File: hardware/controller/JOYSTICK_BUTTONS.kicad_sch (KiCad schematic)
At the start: 14 parts, among them J2 Joystick, J3 Joystick, SW1 UP, SW2 LEFT, SW3 DOWN, SW4 RGHT, SW5 BOOT, SW6 RESET

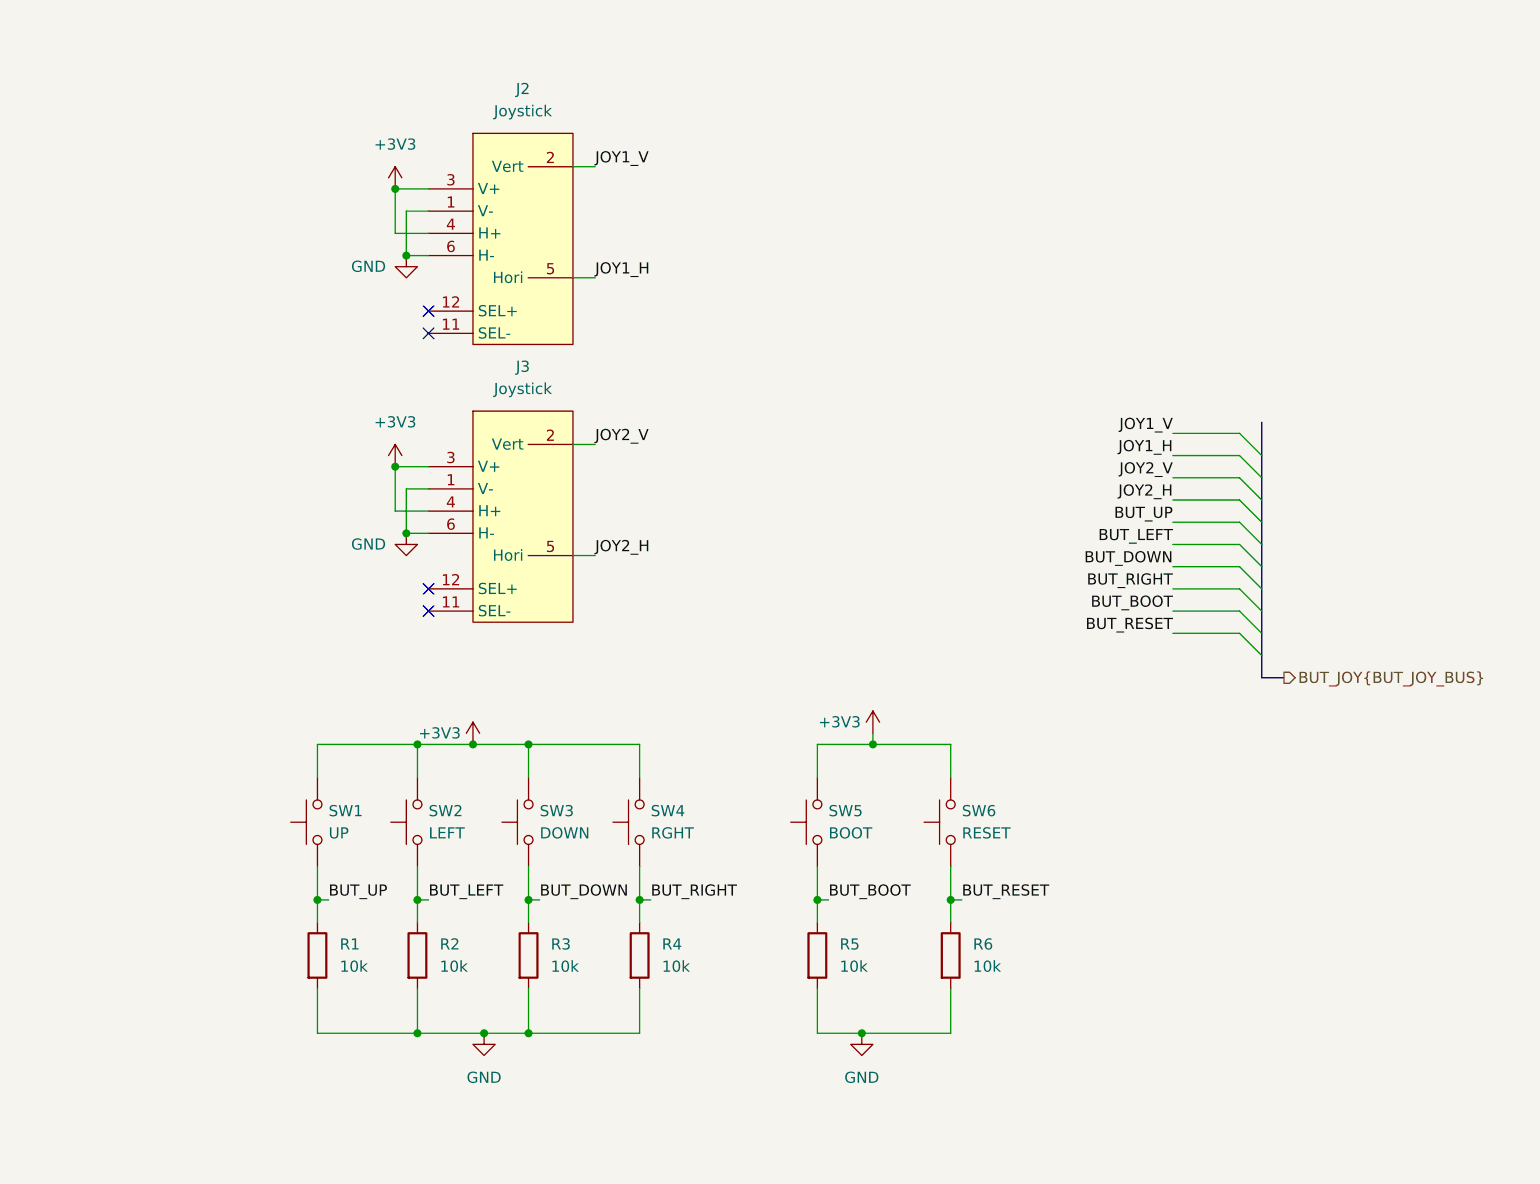
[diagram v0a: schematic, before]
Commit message: fixed bus stuff
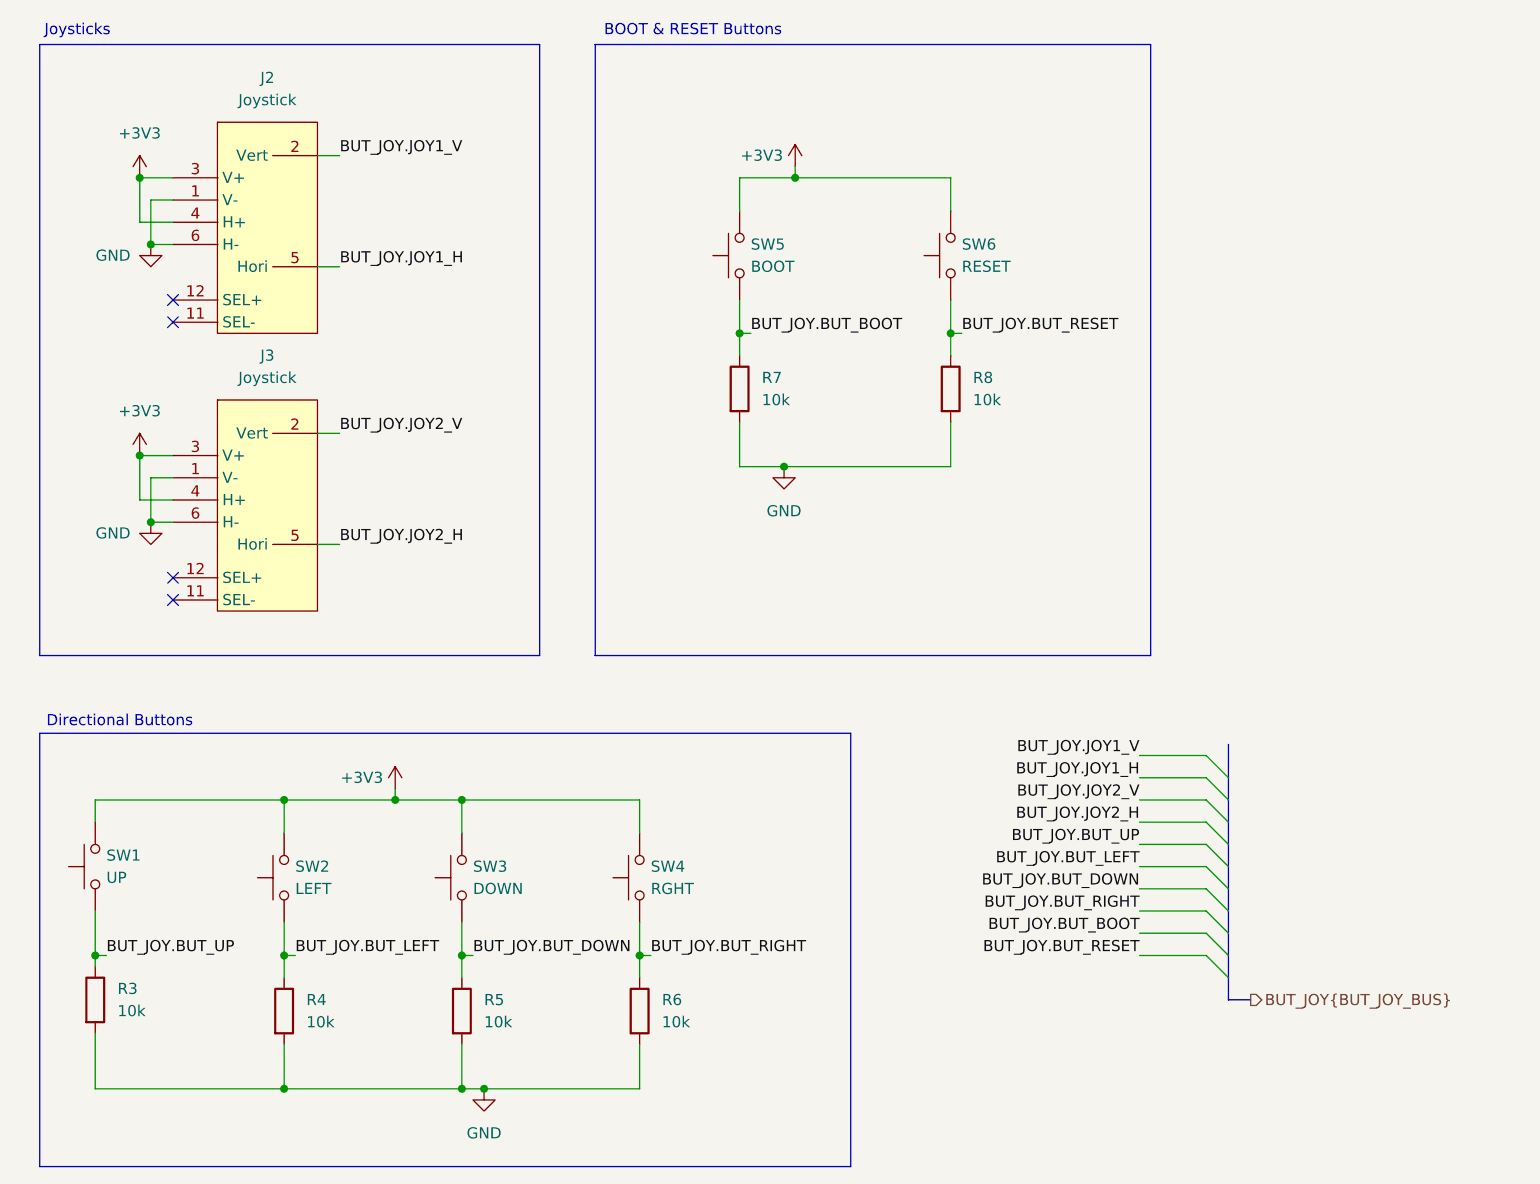
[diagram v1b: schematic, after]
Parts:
- renumbered R1 to R3, R2 to R4, R3 to R5, R4 to R6, R5 to R7, R6 to R8
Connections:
- net BUT_BOOT renamed BUT_JOY.BUT_BOOT
- net BUT_DOWN renamed BUT_JOY.BUT_DOWN
- net BUT_LEFT renamed BUT_JOY.BUT_LEFT
- net BUT_RESET renamed BUT_JOY.BUT_RESET
- net BUT_RIGHT renamed BUT_JOY.BUT_RIGHT
- net BUT_UP renamed BUT_JOY.BUT_UP
- net JOY1_H renamed BUT_JOY.JOY1_H
- net JOY1_V renamed BUT_JOY.JOY1_V
- net JOY2_H renamed BUT_JOY.JOY2_H
- net JOY2_V renamed BUT_JOY.JOY2_V
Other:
- note added: "BOOT & RESET Buttons"
- note added: "Directional Buttons"
- note added: "Joysticks"
- moved on the sheet: J2, J3, R3, R4, R5, R6, R7, R8, SW1, SW2, SW3, SW4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
